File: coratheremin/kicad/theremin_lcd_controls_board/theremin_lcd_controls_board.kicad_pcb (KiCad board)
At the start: 2 copper layers, 222.2 x 80 mm, 88 parts, among them J1 Encoders, J2 Pots ADC, SW1 EC11E, SW2 EC11E, SW3 EC11E, SW4 EC11E, SW5 EC11E, SW6 EC11E, SW7 EC11E, SW8 EC11E, U1 74HC165, U2 74HC165, U3 74HC165, U4 MCP3208

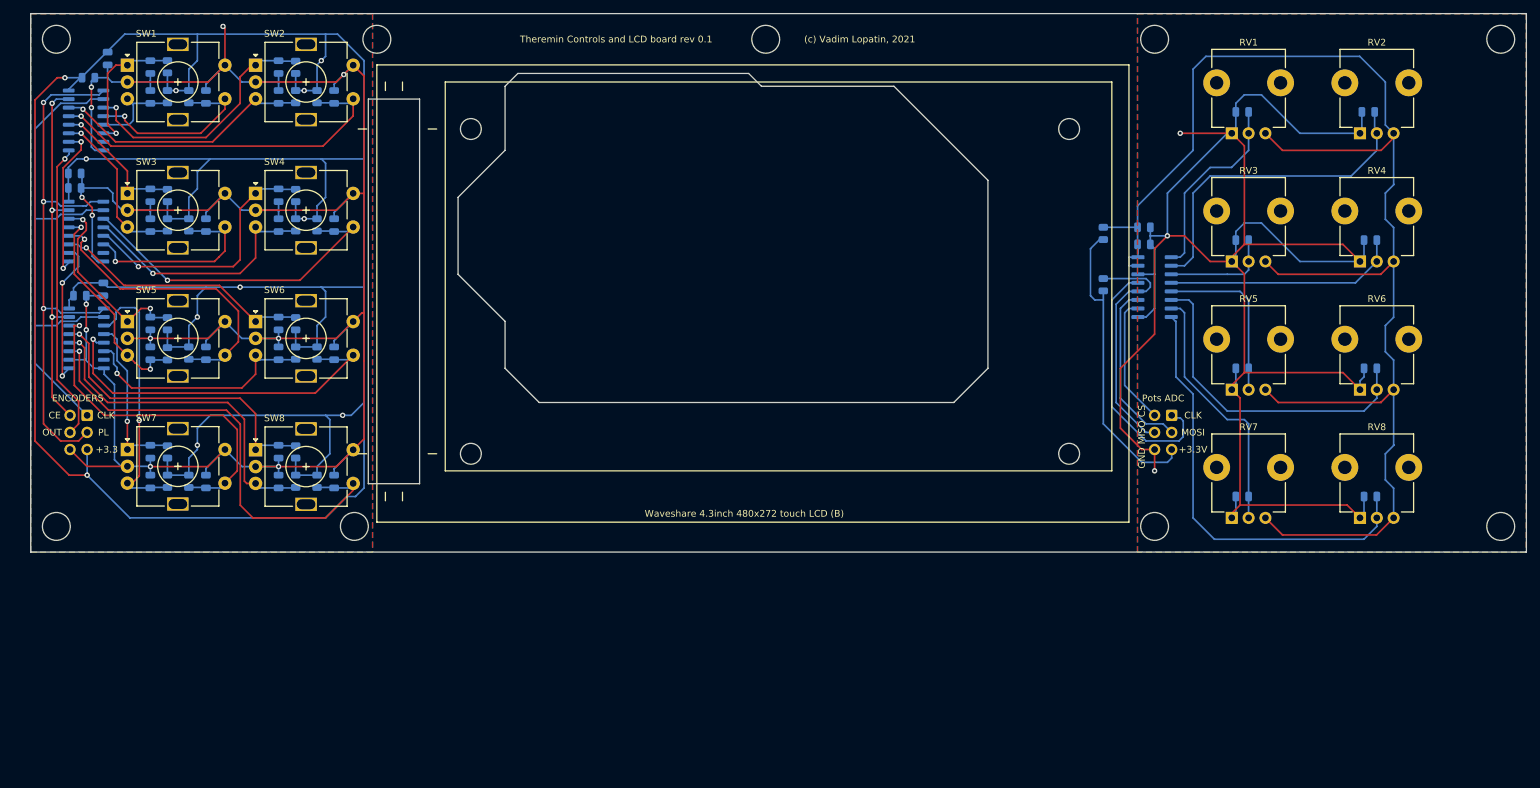
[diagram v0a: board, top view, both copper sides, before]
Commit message: pcbs updated, jlcpcb prod rev 0.1, gerber files
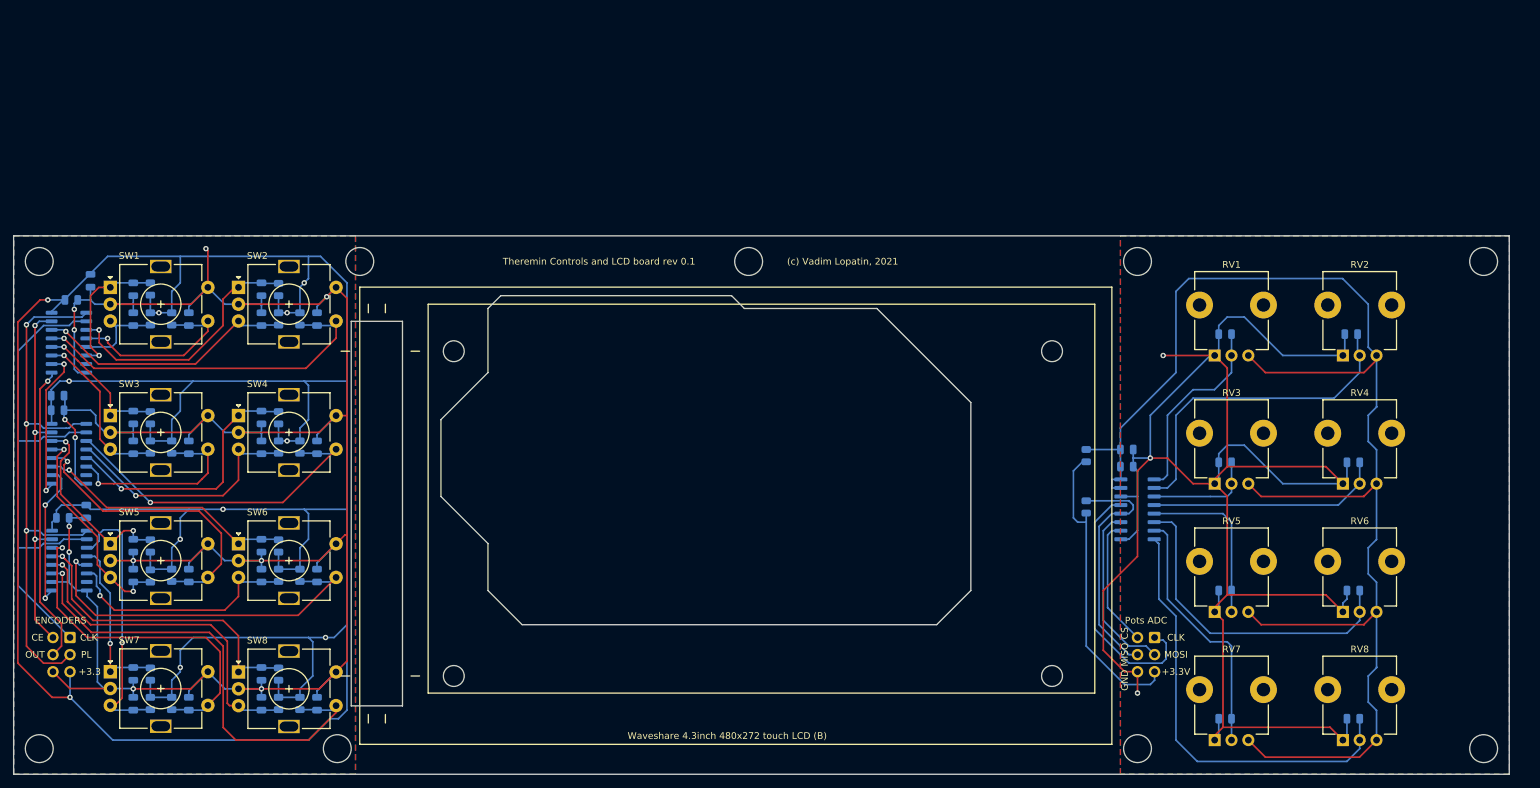
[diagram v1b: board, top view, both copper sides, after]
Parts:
- moved C35 33.1 mm to (212.4, 118.7)
- moved C36 33.1 mm to (231.5, 118.7)
- moved C40 33.1 mm to (197.8, 97.8)
- moved J1 33.1 mm to (40.8, 125.7)
- moved J2 33.1 mm to (201.9, 125.7)
- moved R11 33.1 mm to (71.8, 97.4)
- moved R12 33.1 mm to (74.9, 97.4)
- moved R13 33.1 mm to (52.7, 112.1)
- moved R16 33.1 mm to (71.8, 112.1)
- moved R26 33.1 mm to (191.8, 106.3)
- moved R8 33.1 mm to (52.7, 97.4)
- moved R9 33.1 mm to (55.9, 97.4)
- moved RV3 33.1 mm to (210.9, 102.9)
- moved RV4 33.1 mm to (229.9, 102.9)
- moved U4 33.1 mm to (199.4, 106.7)
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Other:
- outline, holes or cut-outs redrawn
